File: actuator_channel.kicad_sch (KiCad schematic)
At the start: 6 parts, among them U1 DRV8871 H-мост

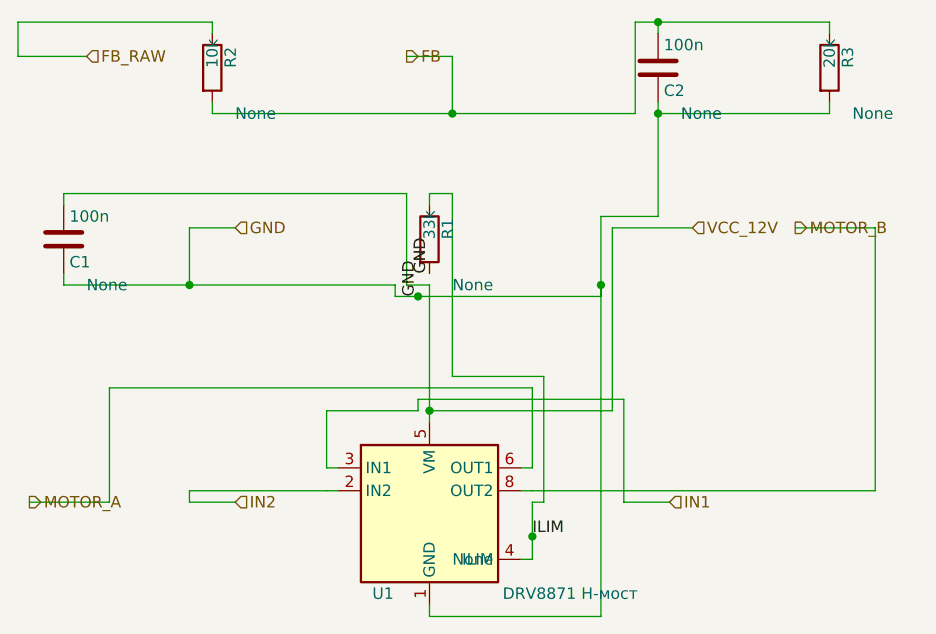
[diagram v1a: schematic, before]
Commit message: refactoring
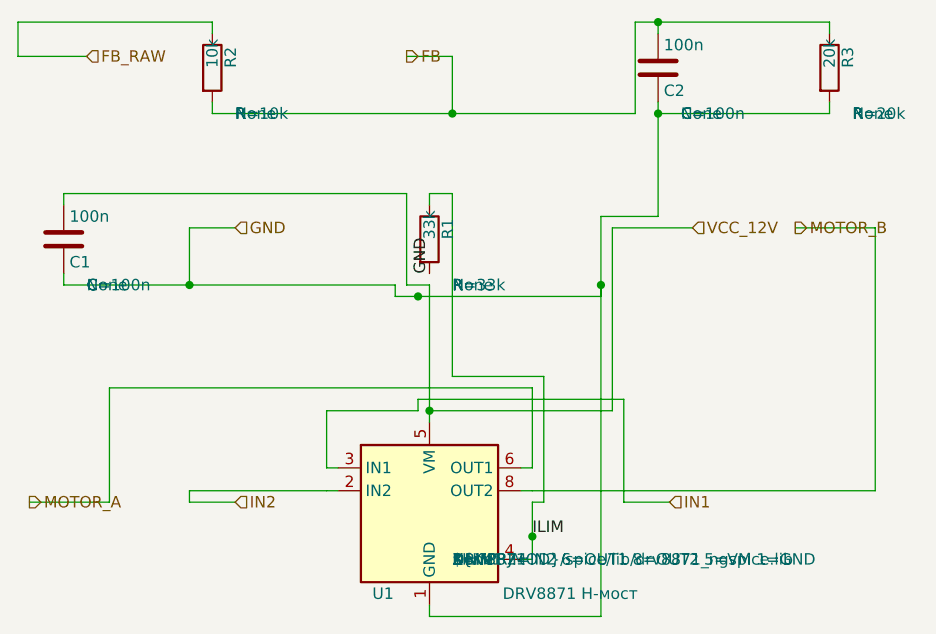
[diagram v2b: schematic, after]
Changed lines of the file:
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@@
+			)
+		)
+		(property "Sim.Device" "X"
+			(at 50.8 62.2299 0)
+			(effects
+				(font
+					(size 1.27 1.27)
+				)
+				(justify left)
+			)
+		)
+		(property "Sim.Name" "DRV8871"
+			(at 50.8 62.2299 0)
+			(effects
+				(font
+					(size 1.27 1.27)
+				)
+				(justify left)
+			)
+		)
+		(property "Sim.Library" "${KIPRJMOD}/spice/lib/drv8871_ngspice.lib"
+			(at 50.8 62.2299 0)
+			(effects
+				(font
+					(size 1.27 1.27)
+				)
+				(justify left)
+			)
+		)
+		(property "Sim.Pins" "3=IN1 2=IN2 6=OUT1 8=OUT2 5=VM 1=GND"
+			(at 50.8 62.2299 0)
+			(effects
+				(font
+					(size 1.27 1.27)
+				)
+				(justify left)
+			)
+		)
+		(property "Sim.Enable" "1"
+			(at 50.8 62.2299 0)
+			(effects
+				(font
+					(size 1.27 1.27)
+				)
+				(justify left)
 			)
 		)
@@
 		(instances
 			(project "climate_control_niva_travel"
-				(path "/165a98f1-2dde-4141-9fdc-c935d39c8cff/71043f52-0d77-45aa-8712-29726f06dba9/"
+				(path "/cc416b40-1361-4232-ac1e-5cd36ef0c0fb/00d495cc-b649-406c-a770-8fe368be32b1/"
 					(reference "U1101")
 					(unit 1)
@@
 			)
 			(project "climate_control_niva_travel"
-				(path "/165a98f1-2dde-4141-9fdc-c935d39c8cff/2f3ffc4a-2693-497f-8d4f-33350471cfa5/"
+				(path "/cc416b40-1361-4232-ac1e-5cd36ef0c0fb/c7763710-e92c-4c28-a886-41af9165c1e6/"
 					(reference "U1201")
 					(unit 1)
@@
 			)
 			(project "climate_control_niva_travel"
-				(path "/165a98f1-2dde-4141-9fdc-c935d39c8cff/9a28178d-7623-4d94-ab78-dd6c6870fb3e/"
+				(path "/cc416b40-1361-4232-ac1e-5cd36ef0c0fb/d129c75d-f93c-4933-9b30-a4a7cbaa20f2/"
 					(reference "U1301")
 					(unit 1)
@@
 			)
 			(project "climate_control_niva_travel"
-				(path "/165a98f1-2dde-4141-9fdc-c935d39c8cff/066dde15-4272-4ac0-97f9-736df0d6b182/"
+				(path "/cc416b40-1361-4232-ac1e-5cd36ef0c0fb/725528c8-ac11-49bd-9902-814aea31595d/"
 					(reference "U1401")
 					(unit 1)
@@
 			)
 		)
+		(property "Sim.Device" "C"
+			(at 10.16 31.7499 0)
+			(effects
+				(font
+					(size 1.27 1.27)
+				)
+				(justify left)
+			)
+		)
+		(property "Sim.Params" "C=100n"
+			(at 10.16 31.7499 0)
+			(effects
+				(font
+					(size 1.27 1.27)
+				)
+				(justify left)
+			)
+		)
 		(pin "1"
 		)
@@
 		(instances
 			(project "climate_control_niva_travel"
-				(path "/165a98f1-2dde-4141-9fdc-c935d39c8cff/71043f52-0d77-45aa-8712-29726f06dba9/"
+				(path "/cc416b40-1361-4232-ac1e-5cd36ef0c0fb/00d495cc-b649-406c-a770-8fe368be32b1/"
 					(reference "C1101")
 					(unit 1)
@@
 			)
 			(project "climate_control_niva_travel"
-				(path "/165a98f1-2dde-4141-9fdc-c935d39c8cff/2f3ffc4a-2693-497f-8d4f-33350471cfa5/"
+				(path "/cc416b40-1361-4232-ac1e-5cd36ef0c0fb/c7763710-e92c-4c28-a886-41af9165c1e6/"
 					(reference "C1201")
 					(unit 1)
@@
 			)
 			(project "climate_control_niva_travel"
-				(path "/165a98f1-2dde-4141-9fdc-c935d39c8cff/9a28178d-7623-4d94-ab78-dd6c6870fb3e/"
+				(path "/cc416b40-1361-4232-ac1e-5cd36ef0c0fb/d129c75d-f93c-4933-9b30-a4a7cbaa20f2/"
 					(reference "C1301")
 					(unit 1)
@@
 			)
 			(project "climate_control_niva_travel"
-				(path "/165a98f1-2dde-4141-9fdc-c935d39c8cff/066dde15-4272-4ac0-97f9-736df0d6b182/"
+				(path "/cc416b40-1361-4232-ac1e-5cd36ef0c0fb/725528c8-ac11-49bd-9902-814aea31595d/"
 					(reference "C1401")
 					(unit 1)
@@
 			)
 		)
+		(property "Sim.Device" "R"
+			(at 50.8 31.7499 0)
+			(effects
+				(font
+					(size 1.27 1.27)
+				)
+				(justify left)
+			)
+		)
+		(property "Sim.Params" "R=33k"
+			(at 50.8 31.7499 0)
+			(effects
+				(font
+					(size 1.27 1.27)
+				)
+				(justify left)
+			)
+		)
 		(pin "1"
 		)
@@
 		(instances
 			(project "climate_control_niva_travel"
-				(path "/165a98f1-2dde-4141-9fdc-c935d39c8cff/71043f52-0d77-45aa-8712-29726f06dba9/"
+				(path "/cc416b40-1361-4232-ac1e-5cd36ef0c0fb/00d495cc-b649-406c-a770-8fe368be32b1/"
 					(reference "R1101")
 					(unit 1)
@@
 			)
 			(project "climate_control_niva_travel"
-				(path "/165a98f1-2dde-4141-9fdc-c935d39c8cff/2f3ffc4a-2693-497f-8d4f-33350471cfa5/"
+				(path "/cc416b40-1361-4232-ac1e-5cd36ef0c0fb/c7763710-e92c-4c28-a886-41af9165c1e6/"
 					(reference "R1201")
 					(unit 1)
@@
 			)
 			(project "climate_control_niva_travel"
-				(path "/165a98f1-2dde-4141-9fdc-c935d39c8cff/9a28178d-7623-4d94-ab78-dd6c6870fb3e/"
+				(path "/cc416b40-1361-4232-ac1e-5cd36ef0c0fb/d129c75d-f93c-4933-9b30-a4a7cbaa20f2/"
 					(reference "R1301")
 					(unit 1)
@@
 			)
 			(project "climate_control_niva_travel"
-				(path "/165a98f1-2dde-4141-9fdc-c935d39c8cff/066dde15-4272-4ac0-97f9-736df0d6b182/"
+				(path "/cc416b40-1361-4232-ac1e-5cd36ef0c0fb/725528c8-ac11-49bd-9902-814aea31595d/"
 					(reference "R1401")
 					(unit 1)
@@
 			)
 		)
+		(property "Sim.Device" "R"
+			(at 26.67 12.6999 0)
+			(effects
+				(font
+					(size 1.27 1.27)
+				)
+				(justify left)
+			)
+		)
+		(property "Sim.Params" "R=10k"
+			(at 26.67 12.6999 0)
+			(effects
+				(font
+					(size 1.27 1.27)
+				)
+				(justify left)
+			)
+		)
 		(pin "1"
 		)
@@
 		(instances
 			(project "climate_control_niva_travel"
-				(path "/165a98f1-2dde-4141-9fdc-c935d39c8cff/71043f52-0d77-45aa-8712-29726f06dba9/"
+				(path "/cc416b40-1361-4232-ac1e-5cd36ef0c0fb/00d495cc-b649-406c-a770-8fe368be32b1/"
 					(reference "R1102")
 					(unit 1)
@@
 			)
 			(project "climate_control_niva_travel"
-				(path "/165a98f1-2dde-4141-9fdc-c935d39c8cff/2f3ffc4a-2693-497f-8d4f-33350471cfa5/"
+				(path "/cc416b40-1361-4232-ac1e-5cd36ef0c0fb/c7763710-e92c-4c28-a886-41af9165c1e6/"
 					(reference "R1202")
 					(unit 1)
@@
 			)
 			(project "climate_control_niva_travel"
-				(path "/165a98f1-2dde-4141-9fdc-c935d39c8cff/9a28178d-7623-4d94-ab78-dd6c6870fb3e/"
+				(path "/cc416b40-1361-4232-ac1e-5cd36ef0c0fb/d129c75d-f93c-4933-9b30-a4a7cbaa20f2/"
 					(reference "R1302")
 					(unit 1)
@@
 			)
 			(project "climate_control_niva_travel"
-				(path "/165a98f1-2dde-4141-9fdc-c935d39c8cff/066dde15-4272-4ac0-97f9-736df0d6b182/"
+				(path "/cc416b40-1361-4232-ac1e-5cd36ef0c0fb/725528c8-ac11-49bd-9902-814aea31595d/"
 					(reference "R1402")
 					(unit 1)
@@
 			)
 		)
+		(property "Sim.Device" "R"
+			(at 95.25 12.6999 0)
+			(effects
+				(font
+					(size 1.27 1.27)
+				)
+				(justify left)
+			)
+		)
+		(property "Sim.Params" "R=20k"
+			(at 95.25 12.6999 0)
+			(effects
+				(font
+					(size 1.27 1.27)
+				)
+				(justify left)
+			)
+		)
 		(pin "1"
 		)
@@
 		(instances
 			(project "climate_control_niva_travel"
-				(path "/165a98f1-2dde-4141-9fdc-c935d39c8cff/71043f52-0d77-45aa-8712-29726f06dba9/"
+				(path "/cc416b40-1361-4232-ac1e-5cd36ef0c0fb/00d495cc-b649-406c-a770-8fe368be32b1/"
 					(reference "R1103")
 					(unit 1)
@@
 			)
 			(project "climate_control_niva_travel"
-				(path "/165a98f1-2dde-4141-9fdc-c935d39c8cff/2f3ffc4a-2693-497f-8d4f-33350471cfa5/"
+				(path "/cc416b40-1361-4232-ac1e-5cd36ef0c0fb/c7763710-e92c-4c28-a886-41af9165c1e6/"
 					(reference "R1203")
 					(unit 1)
@@
 			)
 			(project "climate_control_niva_travel"
-				(path "/165a98f1-2dde-4141-9fdc-c935d39c8cff/9a28178d-7623-4d94-ab78-dd6c6870fb3e/"
+				(path "/cc416b40-1361-4232-ac1e-5cd36ef0c0fb/d129c75d-f93c-4933-9b30-a4a7cbaa20f2/"
 					(reference "R1303")
 					(unit 1)
@@
 			)
 			(project "climate_control_niva_travel"
-				(path "/165a98f1-2dde-4141-9fdc-c935d39c8cff/066dde15-4272-4ac0-97f9-736df0d6b182/"
+				(path "/cc416b40-1361-4232-ac1e-5cd36ef0c0fb/725528c8-ac11-49bd-9902-814aea31595d/"
 					(reference "R1403")
 					(unit 1)
@@
 			)
 		)
+		(property "Sim.Device" "C"
+			(at 76.2 12.6999 0)
+			(effects
+				(font
+					(size 1.27 1.27)
+				)
+				(justify left)
+			)
+		)
+		(property "Sim.Params" "C=100n"
+			(at 76.2 12.6999 0)
+			(effects
+				(font
+					(size 1.27 1.27)
+				)
+				(justify left)
+			)
+		)
 		(pin "1"
 		)
@@
 		(instances
 			(project "climate_control_niva_travel"
-				(path "/165a98f1-2dde-4141-9fdc-c935d39c8cff/71043f52-0d77-45aa-8712-29726f06dba9/"
+				(path "/cc416b40-1361-4232-ac1e-5cd36ef0c0fb/00d495cc-b649-406c-a770-8fe368be32b1/"
 					(reference "C1102")
 					(unit 1)
@@
 			)
 			(project "climate_control_niva_travel"
-				(path "/165a98f1-2dde-4141-9fdc-c935d39c8cff/2f3ffc4a-2693-497f-8d4f-33350471cfa5/"
+				(path "/cc416b40-1361-4232-ac1e-5cd36ef0c0fb/c7763710-e92c-4c28-a886-41af9165c1e6/"
 					(reference "C1202")
 					(unit 1)
@@
 			)
 			(project "climate_control_niva_travel"
-				(path "/165a98f1-2dde-4141-9fdc-c935d39c8cff/9a28178d-7623-4d94-ab78-dd6c6870fb3e/"
+				(path "/cc416b40-1361-4232-ac1e-5cd36ef0c0fb/d129c75d-f93c-4933-9b30-a4a7cbaa20f2/"
 					(reference "C1302")
 					(unit 1)
@@
 			)
 			(project "climate_control_niva_travel"
-				(path "/165a98f1-2dde-4141-9fdc-c935d39c8cff/066dde15-4272-4ac0-97f9-736df0d6b182/"
+				(path "/cc416b40-1361-4232-ac1e-5cd36ef0c0fb/725528c8-ac11-49bd-9902-814aea31595d/"
 					(reference "C1402")
 					(unit 1)
@@
 	(junction
 		(at 48.26 45.72)
-		(diameter 0)
+		(diameter 0.0000)
 		(color 0 0 0 0)
 	)
 	(junction
 		(at 73.66 12.7)
-		(diameter 0)
+		(diameter 0.0000)
 		(color 0 0 0 0)
 	)
 	(junction
 		(at 67.31 31.75)
-		(diameter 0)
+		(diameter 0.0000)
 		(color 0 0 0 0)
 	)
 	(junction
 		(at 46.99 33.02)
-		(diameter 0)
+		(diameter 0.0000)
 		(color 0 0 0 0)
 	)
 	(junction
 		(at 21.59 31.75)
-		(diameter 0)
+		(diameter 0.0000)
 		(color 0 0 0 0)
 	)
 	(junction
 		(at 73.66 2.54)
-		(diameter 0)
+		(diameter 0.0000)
 		(color 0 0 0 0)
 	)
 	(junction
 		(at 50.8 12.7)
-		(diameter 0)
+		(diameter 0.0000)
 		(color 0 0 0 0)
 	)
 	(junction
 		(at 59.69 59.69)
-		(diameter 0)
+		(diameter 0.0000)
 		(color 0 0 0 0)
 	)
@@
 		(effects
 			(font
-				(size 1.27 1.27)
-			)
-			(justify left bottom)
-		)
-	)
-	(label "GND"
-		(at 46.99 33.02 270)
-		(effects
-			(font

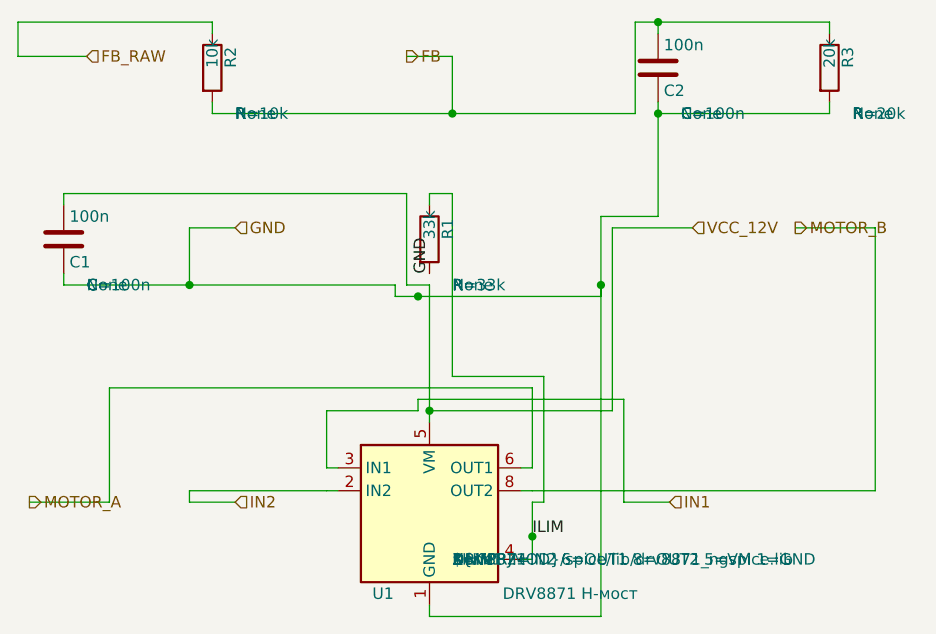
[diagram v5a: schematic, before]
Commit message: fix
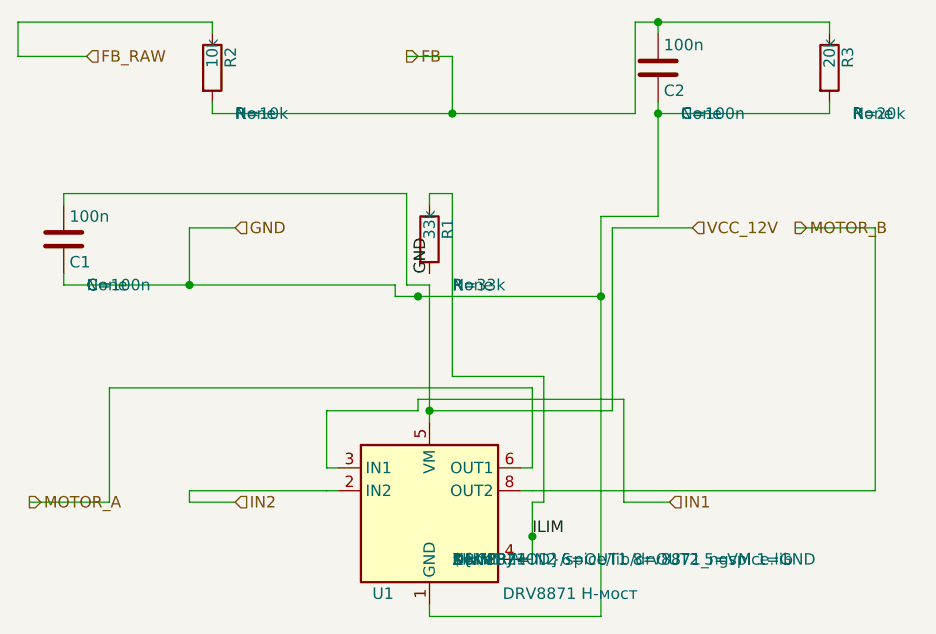
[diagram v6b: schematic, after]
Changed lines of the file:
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@@
 				(instances
 			(project "climate_control_niva_travel"
-				(path "/a20a8d43-2e18-4318-8ef3-7f434a470dab/fb0f2749-c662-4061-8cce-0319f035f1a8"(reference "U1101") (unit 1) )
-				(path "/a20a8d43-2e18-4318-8ef3-7f434a470dab/3ddf28b5-d77b-42d1-9e28-06c757bc079d"(reference "U1201") (unit 1) )
-				(path "/a20a8d43-2e18-4318-8ef3-7f434a470dab/e2c6e160-3bfb-4c58-8e68-e8b3df657076"(reference "U1301") (unit 1) )
-				(path "/a20a8d43-2e18-4318-8ef3-7f434a470dab/71c49532-965c-4bbc-bb04-9de7ab700f7e"(reference "U1401") (unit 1) )
+				(path "/a57a4e28-3e5b-4632-bf9b-60d8c206f50d"(reference "U1") (unit 1) )
+				(path "/aece091b-8e26-4b21-9786-1b0efc647a51/9de855ac-423f-43f9-81ec-14f73972ce86"(reference "U1101") (unit 1) )
+				(path "/aece091b-8e26-4b21-9786-1b0efc647a51/0ae41e85-00a1-4547-afdb-bf1155e791a4"(reference "U1201") (unit 1) )
+				(path "/aece091b-8e26-4b21-9786-1b0efc647a51/61cbfd25-d0a0-47d9-baa4-5d4111a0d1c4"(reference "U1301") (unit 1) )
+				(path "/aece091b-8e26-4b21-9786-1b0efc647a51/fbc42ef4-6473-4ce0-b625-0ecd1256b71b"(reference "U1401") (unit 1) )
 			)
 		)
@@
 				(instances
 			(project "climate_control_niva_travel"
-				(path "/a20a8d43-2e18-4318-8ef3-7f434a470dab/fb0f2749-c662-4061-8cce-0319f035f1a8"(reference "C1101") (unit 1) )
-				(path "/a20a8d43-2e18-4318-8ef3-7f434a470dab/3ddf28b5-d77b-42d1-9e28-06c757bc079d"(reference "C1201") (unit 1) )
-				(path "/a20a8d43-2e18-4318-8ef3-7f434a470dab/e2c6e160-3bfb-4c58-8e68-e8b3df657076"(reference "C1301") (unit 1) )
-				(path "/a20a8d43-2e18-4318-8ef3-7f434a470dab/71c49532-965c-4bbc-bb04-9de7ab700f7e"(reference "C1401") (unit 1) )
+				(path "/a57a4e28-3e5b-4632-bf9b-60d8c206f50d"(reference "C1") (unit 1) )
+				(path "/aece091b-8e26-4b21-9786-1b0efc647a51/9de855ac-423f-43f9-81ec-14f73972ce86"(reference "C1101") (unit 1) )
+				(path "/aece091b-8e26-4b21-9786-1b0efc647a51/0ae41e85-00a1-4547-afdb-bf1155e791a4"(reference "C1201") (unit 1) )
+				(path "/aece091b-8e26-4b21-9786-1b0efc647a51/61cbfd25-d0a0-47d9-baa4-5d4111a0d1c4"(reference "C1301") (unit 1) )
+				(path "/aece091b-8e26-4b21-9786-1b0efc647a51/fbc42ef4-6473-4ce0-b625-0ecd1256b71b"(reference "C1401") (unit 1) )
 			)
 		)
@@
 				(instances
 			(project "climate_control_niva_travel"
-				(path "/a20a8d43-2e18-4318-8ef3-7f434a470dab/fb0f2749-c662-4061-8cce-0319f035f1a8"(reference "R1101") (unit 1) )
-				(path "/a20a8d43-2e18-4318-8ef3-7f434a470dab/3ddf28b5-d77b-42d1-9e28-06c757bc079d"(reference "R1201") (unit 1) )
-				(path "/a20a8d43-2e18-4318-8ef3-7f434a470dab/e2c6e160-3bfb-4c58-8e68-e8b3df657076"(reference "R1301") (unit 1) )
-				(path "/a20a8d43-2e18-4318-8ef3-7f434a470dab/71c49532-965c-4bbc-bb04-9de7ab700f7e"(reference "R1401") (unit 1) )
+				(path "/a57a4e28-3e5b-4632-bf9b-60d8c206f50d"(reference "R1") (unit 1) )
+				(path "/aece091b-8e26-4b21-9786-1b0efc647a51/9de855ac-423f-43f9-81ec-14f73972ce86"(reference "R1101") (unit 1) )
+				(path "/aece091b-8e26-4b21-9786-1b0efc647a51/0ae41e85-00a1-4547-afdb-bf1155e791a4"(reference "R1201") (unit 1) )
+				(path "/aece091b-8e26-4b21-9786-1b0efc647a51/61cbfd25-d0a0-47d9-baa4-5d4111a0d1c4"(reference "R1301") (unit 1) )
+				(path "/aece091b-8e26-4b21-9786-1b0efc647a51/fbc42ef4-6473-4ce0-b625-0ecd1256b71b"(reference "R1401") (unit 1) )
 			)
 		)
@@
 				(instances
 			(project "climate_control_niva_travel"
-				(path "/a20a8d43-2e18-4318-8ef3-7f434a470dab/fb0f2749-c662-4061-8cce-0319f035f1a8"(reference "R1102") (unit 1) )
-				(path "/a20a8d43-2e18-4318-8ef3-7f434a470dab/3ddf28b5-d77b-42d1-9e28-06c757bc079d"(reference "R1202") (unit 1) )
-				(path "/a20a8d43-2e18-4318-8ef3-7f434a470dab/e2c6e160-3bfb-4c58-8e68-e8b3df657076"(reference "R1302") (unit 1) )
-				(path "/a20a8d43-2e18-4318-8ef3-7f434a470dab/71c49532-965c-4bbc-bb04-9de7ab700f7e"(reference "R1402") (unit 1) )
+				(path "/a57a4e28-3e5b-4632-bf9b-60d8c206f50d"(reference "R2") (unit 1) )
+				(path "/aece091b-8e26-4b21-9786-1b0efc647a51/9de855ac-423f-43f9-81ec-14f73972ce86"(reference "R1102") (unit 1) )
+				(path "/aece091b-8e26-4b21-9786-1b0efc647a51/0ae41e85-00a1-4547-afdb-bf1155e791a4"(reference "R1202") (unit 1) )
+				(path "/aece091b-8e26-4b21-9786-1b0efc647a51/61cbfd25-d0a0-47d9-baa4-5d4111a0d1c4"(reference "R1302") (unit 1) )
+				(path "/aece091b-8e26-4b21-9786-1b0efc647a51/fbc42ef4-6473-4ce0-b625-0ecd1256b71b"(reference "R1402") (unit 1) )
 			)
 		)
@@
 				(instances
 			(project "climate_control_niva_travel"
-				(path "/a20a8d43-2e18-4318-8ef3-7f434a470dab/fb0f2749-c662-4061-8cce-0319f035f1a8"(reference "R1103") (unit 1) )
-				(path "/a20a8d43-2e18-4318-8ef3-7f434a470dab/3ddf28b5-d77b-42d1-9e28-06c757bc079d"(reference "R1203") (unit 1) )
-				(path "/a20a8d43-2e18-4318-8ef3-7f434a470dab/e2c6e160-3bfb-4c58-8e68-e8b3df657076"(reference "R1303") (unit 1) )
-				(path "/a20a8d43-2e18-4318-8ef3-7f434a470dab/71c49532-965c-4bbc-bb04-9de7ab700f7e"(reference "R1403") (unit 1) )
+				(path "/a57a4e28-3e5b-4632-bf9b-60d8c206f50d"(reference "R3") (unit 1) )
+				(path "/aece091b-8e26-4b21-9786-1b0efc647a51/9de855ac-423f-43f9-81ec-14f73972ce86"(reference "R1103") (unit 1) )
+				(path "/aece091b-8e26-4b21-9786-1b0efc647a51/0ae41e85-00a1-4547-afdb-bf1155e791a4"(reference "R1203") (unit 1) )
+				(path "/aece091b-8e26-4b21-9786-1b0efc647a51/61cbfd25-d0a0-47d9-baa4-5d4111a0d1c4"(reference "R1303") (unit 1) )
+				(path "/aece091b-8e26-4b21-9786-1b0efc647a51/fbc42ef4-6473-4ce0-b625-0ecd1256b71b"(reference "R1403") (unit 1) )
 			)
 		)
@@
 				(instances
 			(project "climate_control_niva_travel"
-				(path "/a20a8d43-2e18-4318-8ef3-7f434a470dab/fb0f2749-c662-4061-8cce-0319f035f1a8"(reference "C1102") (unit 1) )
-				(path "/a20a8d43-2e18-4318-8ef3-7f434a470dab/3ddf28b5-d77b-42d1-9e28-06c757bc079d"(reference "C1202") (unit 1) )
-				(path "/a20a8d43-2e18-4318-8ef3-7f434a470dab/e2c6e160-3bfb-4c58-8e68-e8b3df657076"(reference "C1302") (unit 1) )
-				(path "/a20a8d43-2e18-4318-8ef3-7f434a470dab/71c49532-965c-4bbc-bb04-9de7ab700f7e"(reference "C1402") (unit 1) )
+				(path "/a57a4e28-3e5b-4632-bf9b-60d8c206f50d"(reference "C2") (unit 1) )
+				(path "/aece091b-8e26-4b21-9786-1b0efc647a51/9de855ac-423f-43f9-81ec-14f73972ce86"(reference "C1102") (unit 1) )
+				(path "/aece091b-8e26-4b21-9786-1b0efc647a51/0ae41e85-00a1-4547-afdb-bf1155e791a4"(reference "C1202") (unit 1) )
+				(path "/aece091b-8e26-4b21-9786-1b0efc647a51/61cbfd25-d0a0-47d9-baa4-5d4111a0d1c4"(reference "C1302") (unit 1) )
+				(path "/aece091b-8e26-4b21-9786-1b0efc647a51/fbc42ef4-6473-4ce0-b625-0ecd1256b71b"(reference "C1402") (unit 1) )
 			)
 		)
@@
 		(pts
 			(xy 44.45 33.02) (xy 67.31 33.02)
-		)
-		(stroke
-			(width 0)
-			(type default)
-		)
-	)
-	(wire
-		(pts
-			(xy 67.31 33.02) (xy 67.31 31.75)
 		)
 		(stroke
@@
 	)
 	(junction
-		(at 67.31 31.75)
+		(at 67.31 33.02)
 		(diameter 0.0000)
 		(color 0 0 0 0)
